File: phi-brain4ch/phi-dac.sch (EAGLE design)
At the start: 147 parts, among them IC1 PCM1792A, IC10 LM317, IC11 LM337, IC2 OPA1632D, IC3 OPA1632D, IC4 OPA1632D, IC6 OPA1632D, IC7 REG1117-5, IC8 ADP3301ARZ-3.3, IC9 MGJ2D121515SC, J1 CUI-RCJ-2123, J5 DC21P

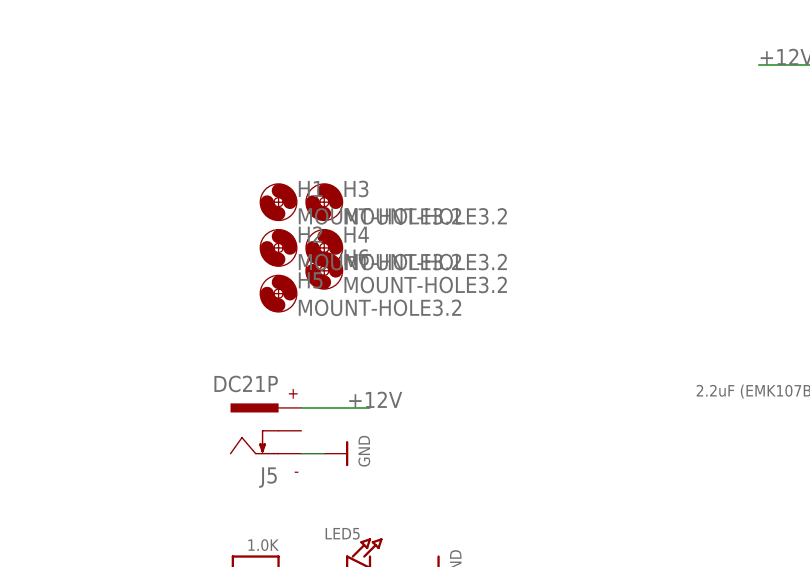
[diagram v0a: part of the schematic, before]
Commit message: routed
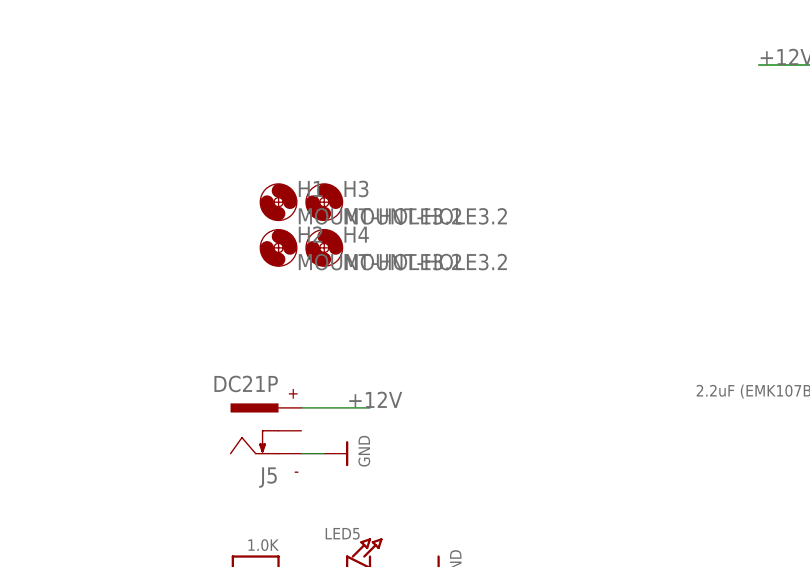
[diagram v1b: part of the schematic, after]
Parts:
- removed H5, H6: MOUNT-HOLE3.2, holes:MOUNT-HOLE3.2
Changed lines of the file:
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@@
 <part name="H1" library="holes" deviceset="MOUNT-HOLE" device="3.2"/>
 <part name="H2" library="holes" deviceset="MOUNT-HOLE" device="3.2"/>
-<part name="H5" library="holes" deviceset="MOUNT-HOLE" device="3.2"/>
-<part name="H6" library="holes" deviceset="MOUNT-HOLE" device="3.2"/>
 <part name="JP1" library="jumper" deviceset="JP4Q" device=""/>
 <part name="R33" library="microbuilder" deviceset="RESISTOR" device="_0805" value="10K 0.1% or better (ERA-3AEB103V)"/>
@@
 <instance part="H1" gate="G$1" x="10.16" y="220.98"/>
 <instance part="H2" gate="G$1" x="10.16" y="215.9"/>
-<instance part="H5" gate="G$1" x="10.16" y="210.82"/>
-<instance part="H6" gate="G$1" x="15.24" y="213.36"/>
 <instance part="JP1" gate="B" x="114.3" y="137.16" rot="R90"/>
 <instance part="R33" gate="G$1" x="144.78" y="132.08"/>

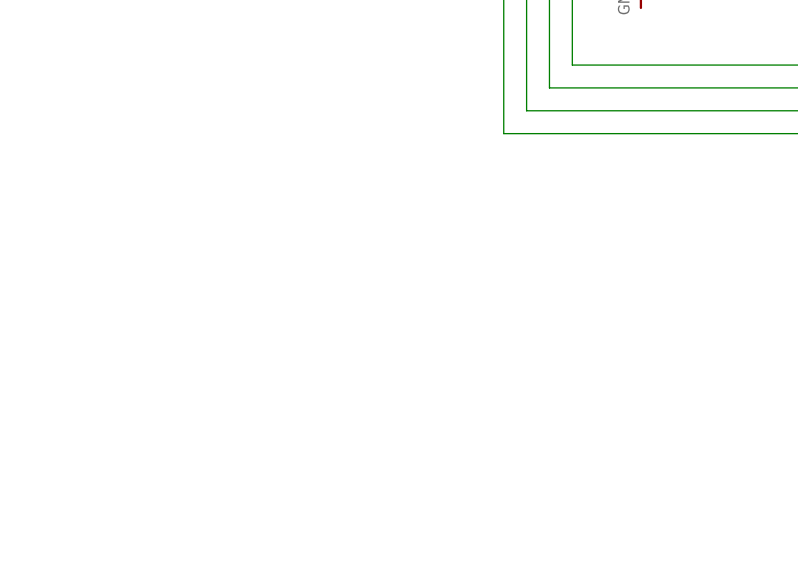
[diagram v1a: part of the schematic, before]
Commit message: routed
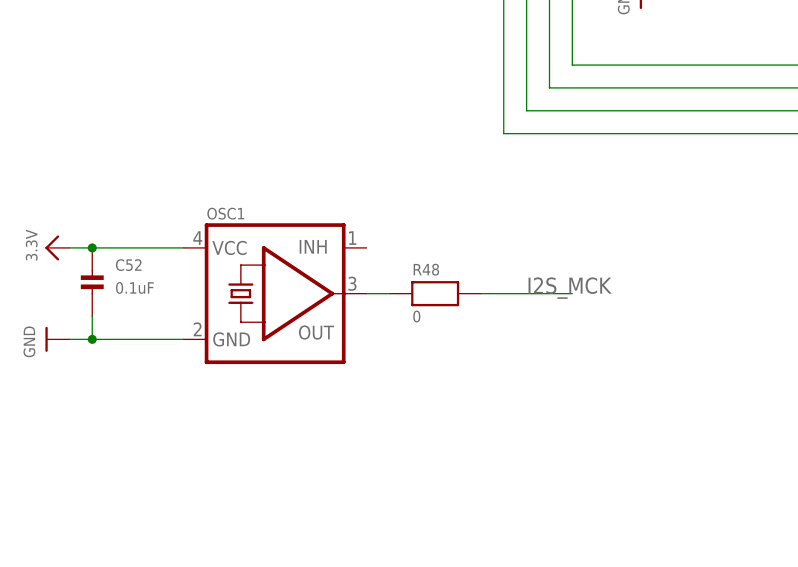
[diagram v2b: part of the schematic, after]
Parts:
- added C52: 0.1uF, microbuilder:CAP_CERAMIC0603
- added OSC1: (no value), microbuilder:OSCILLATOR
- added R48: 0, microbuilder:RESISTOR_0805
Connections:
- new net N$32: OSC1.OUT, R48.1
- net 3.3V: now also C52.P$1, OSC1.VCC
- net GND: now also C52.P$2, OSC1.GND
- net I2S_MCK: now also R48.2
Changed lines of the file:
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@@
 <part name="C50" library="microbuilder" deviceset="CAP_CERAMIC" device="0603" value="0.1u"/>
 <part name="C51" library="microbuilder" deviceset="CAP_CERAMIC" device="1206" value="1uF 12065C105M4Z2A"/>
+<part name="OSC1" library="microbuilder" deviceset="OSCILLATOR" device=""/>
+<part name="C52" library="microbuilder" deviceset="CAP_CERAMIC" device="0603" value="0.1uF"/>
+<part name="U$45" library="microbuilder" deviceset="3.3V" device=""/>
+<part name="U$47" library="microbuilder" deviceset="GND" device=""/>
+<part name="R48" library="microbuilder" deviceset="RESISTOR" device="_0805" value="0"/>
 </parts>
 <sheets>
@@
 <instance part="C50" gate="G$1" x="149.86" y="-12.7"/>
 <instance part="C51" gate="G$1" x="243.84" y="154.94"/>
+<instance part="OSC1" gate="G$1" x="-12.7" y="83.82"/>
+<instance part="C52" gate="G$1" x="-33.02" y="83.82"/>
+<instance part="U$45" gate="G$1" x="-38.1" y="88.9" rot="R90"/>
+<instance part="U$47" gate="G$1" x="-38.1" y="78.74" rot="R270"/>
+<instance part="R48" gate="G$1" x="5.08" y="83.82"/>
 </instances>
 <busses>
@@
 <pinref part="C10" gate="G$1" pin="P$1"/>
 </segment>
+<segment>
+<pinref part="OSC1" gate="G$1" pin="GND"/>
+<pinref part="U$47" gate="G$1" pin="GND"/>
+<wire x1="-22.86" y1="78.74" x2="-33.02" y2="78.74" width="0.1524" layer="91"/>
+<junction x="-33.02" y="78.74"/>
+<wire x1="-33.02" y1="78.74" x2="-35.56" y2="78.74" width="0.1524" layer="91"/>
+<pinref part="C52" gate="G$1" pin="P$2"/>
+<wire x1="-33.02" y1="81.28" x2="-33.02" y2="78.74" width="0.1524" layer="91"/>
+</segment>
 </net>
 <net name="N$1" class="0">
@@
 <wire x1="-5.08" y1="162.56" x2="2.54" y2="162.56" width="0.1524" layer="91"/>
 </segment>
+<segment>
+<pinref part="OSC1" gate="G$1" pin="VCC"/>
+<wire x1="-22.86" y1="88.9" x2="-33.02" y2="88.9" width="0.1524" layer="91"/>
+<pinref part="U$45" gate="G$1" pin="3.3V"/>
+<pinref part="C52" gate="G$1" pin="P$1"/>
+<junction x="-33.02" y="88.9"/>
+<wire x1="-33.02" y1="88.9" x2="-35.56" y2="88.9" width="0.1524" layer="91"/>
+</segment>
 </net>
 <net name="DAC_VCC" class="0">
@@
 <label x="0" y="129.54" size="1.778" layer="95"/>
 <pinref part="SV1" gate="1" pin="9"/>
+</segment>
+<segment>
+<pinref part="R48" gate="G$1" pin="2"/>
+<wire x1="10.16" y1="83.82" x2="20.32" y2="83.82" width="0.1524" layer="91"/>
+<label x="15.24" y="83.82" size="1.778" layer="95"/>
 </segment>
 </net>
@@
 </segment>
 </net>
+<net name="N$32" class="0">
+<segment>
+<pinref part="R48" gate="G$1" pin="1"/>
+<pinref part="OSC1" gate="G$1" pin="OUT"/>
+<wire x1="0" y1="83.82" x2="-2.54" y2="83.82" width="0.1524" layer="91"/>
+</segment>
+</net>
